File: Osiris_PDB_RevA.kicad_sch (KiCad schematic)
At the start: 14 parts, among them J1 BATTERY_IN_4S, J2 ESC1_OUT, J3 ESC2_OUT, J4 ESC3_OUT, J5 ESC4_OUT, J6 OSIRIS_OUT_XT60_M_PIGTAIL

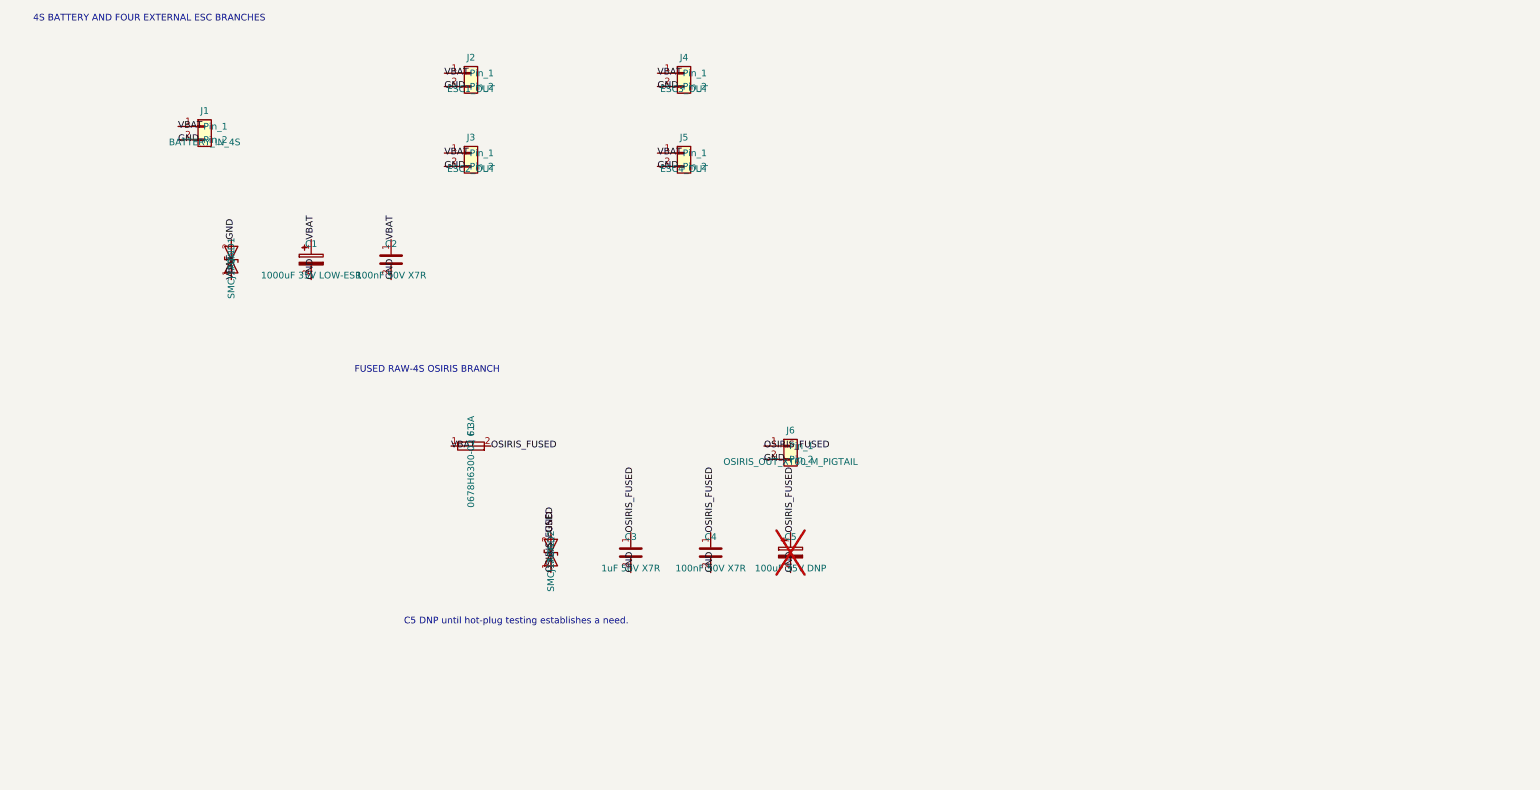
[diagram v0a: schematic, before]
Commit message: FIX
FIX
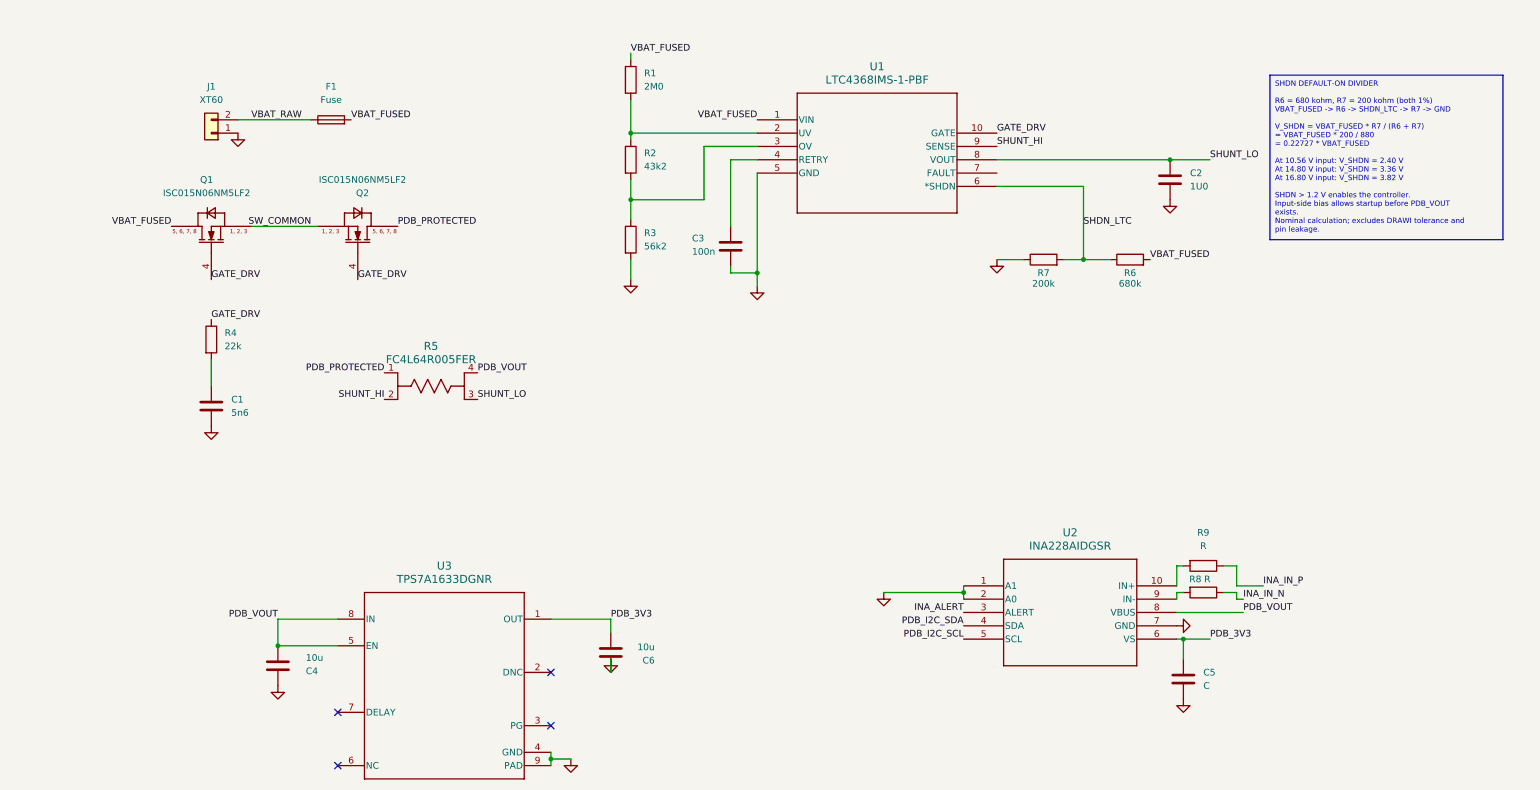
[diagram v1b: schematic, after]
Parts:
- removed C1: 1000uF 35V LOW-ESR, Capacitor_THT:CP_Radial_D12.5mm_P5.00mm, symbol Device:C_Polarized
- removed C5: 100uF 35V DNP, Capacitor_THT:CP_Radial_D8.0mm_P3.50mm, symbol Device:C_Polarized
- removed D1, D2: SMCJ17CA, Diode_SMD:D_SMC, symbol Device:D_TVS
- removed J2: ESC1_OUT, Connector_Wire:SolderWire-4sqmm_1x02_P12mm_D3mm_OD6mm, symbol Connector_Generic:Conn_01x02
- removed J3: ESC2_OUT, Connector_Wire:SolderWire-4sqmm_1x02_P12mm_D3mm_OD6mm, symbol Connector_Generic:Conn_01x02
- removed J4: ESC3_OUT, Connector_Wire:SolderWire-4sqmm_1x02_P12mm_D3mm_OD6mm, symbol Connector_Generic:Conn_01x02
- removed J5: ESC4_OUT, Connector_Wire:SolderWire-4sqmm_1x02_P12mm_D3mm_OD6mm, symbol Connector_Generic:Conn_01x02
- removed J6: OSIRIS_OUT_XT60_M_PIGTAIL, Connector_Wire:SolderWire-2sqmm_1x02_P7.8mm_D2mm_OD3.9mm, symbol Connector_Generic:Conn_01x02
- added C1: 5n6, symbol Device:C
- added C5: C, symbol Device:C
- added C6: 10u, symbol Device:C
- added Q1, Q2: ISC015N06NM5LF2, symbol PDB_Symbols:ISC015N06NM5LF2
- added R1: 2M0, symbol Device:R
- added R2: 43k2, symbol Device:R
- added R3: 56k2, symbol Device:R
- added R4: 22k, symbol Device:R
- added R5: FC4L64R005FER, PDB_Footprints:OH_FC4L64_OHM, symbol PDB_Symbols:FC4L64R005FER
- added R6: 680k, symbol Device:R
- added R7: 200k, symbol Device:R
- added R8, R9: R, symbol Device:R
- added U1: LTC4368IMS-1-PBF, MS_10_ADI, symbol PDB_Symbols:LTC4368IMS-1-PBF
- added U2: INA228AIDGSR, VSSOP10_DGS_TEX, symbol PDB_Symbols:INA228AIDGSR
- added U3: TPS7A1633DGNR, DGN0008C_N, symbol PDB_Symbols:TPS7A1633DGNR
- C2: value 100nF 50V X7R -> 1U0; footprint Capacitor_SMD:C_0805_2012Metric -> (none)
- C3: value 1uF 50V X7R -> 100n; footprint Capacitor_SMD:C_0805_2012Metric -> (none)
- C4: value 100nF 50V X7R -> 10u; footprint Capacitor_SMD:C_0805_2012Metric -> (none)
- F1: value 0678H6300-02 6.3A -> Fuse; footprint PDB_Footprints:FUSC9830X318N -> (none)
- J1: value BATTERY_IN_4S -> XT60; footprint Connector_Wire:SolderWire-4sqmm_1x02_P12mm_D3mm_OD6mm -> (none)
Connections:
- net GND: now also C4.1, J1.1 (Pin_1), C1.2, C5.2, C6.1, R3.2, R7.1, U1.5 (GND), U2.1 (A1), U2.2 (A0), U2.7 (GND), U3.4 (GND), U3.9 (PAD); no longer C4.2, J1.2 (Pin_2)
- removed net OSIRIS_FUSED: C3.1, C4.1, F1.2
- removed net VBAT: C2.1, F1.1, J1.1 (Pin_1)
- new net: C1.1, R4.2
- new net: R9.2, U2.10 (IN+)
- new net: R8.2, U2.9 (IN-)
- new net: R2.2, R3.1, U1.3 (OV)
- new net: R1.2, R2.1, U1.2 (UV)
- new net: C3.1, U1.4 (RETRY)
- new net GATE_DRV: Q1.4 (GATE), Q2.4 (GATE), R4.1, U1.10 (GATE)
- new net INA_ALERT: U2.3 (ALERT)
- new net INA_IN_N: R8.1
- new net INA_IN_P: R9.1
- new net PDB_3V3: C5.1, C6.2, U2.6 (VS), U3.1 (OUT)
- new net PDB_I2C_SCL: U2.5 (SCL)
- new net PDB_I2C_SDA: U2.4 (SDA)
- new net PDB_PROTECTED: Q2.5 (DRAIN), Q2.6 (DRAIN), Q2.7 (DRAIN), Q2.8 (DRAIN), R5.1
- new net PDB_VOUT: C4.2, R5.4, U2.8 (VBUS), U3.5 (EN), U3.8 (IN)
- new net SHDN_LTC: R6.1, R7.2, U1.6 (*SHDN)
- new net SHUNT_HI: R5.2, U1.9 (SENSE)
- new net SHUNT_LO: C2.1, R5.3, U1.8 (VOUT)
- new net SW_COMMON: Q1.1 (SOURCE), Q1.2 (SOURCE), Q1.3 (SOURCE), Q2.1 (SOURCE), Q2.2 (SOURCE), Q2.3 (SOURCE)
- new net VBAT_FUSED: F1.2, Q1.5 (DRAIN), Q1.6 (DRAIN), Q1.7 (DRAIN), Q1.8 (DRAIN), R1.1, R6.2, U1.1 (VIN)
- new net VBAT_RAW: F1.1, J1.2 (Pin_2)
- no-connect marks 0 -> 4
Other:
- note removed: "4S BATTERY AND FOUR EXTERNAL ESC BRANCHES"
- note removed: "C5 DNP until hot-plug testing establishes a need."
- note removed: "FUSED RAW-4S OSIRIS BRANCH"
- company: Osiris UAV -> (none)
- title: Osiris 4S Power Distribution Board -> (none)
